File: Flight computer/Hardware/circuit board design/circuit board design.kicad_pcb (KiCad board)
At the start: 4 copper layers, 30.5 x 82.6 mm, 91 parts, among them J1 Conn_01x05, J2 USB_B_Micro, J3 Screw_Terminal_01x04, J4 Conn_01x02, J5 Screw_Terminal_01x04, J6 Conn_Coaxial, J7 Conn_Coaxial, SW1 SW_DPST, U1 IIS2MDC, U10 BMI088, U11 ATSAML21J18B-AUT, U14 MAX40200AUK, U15 LD3985G33R_TSOT23, U2 0433BM41A0019E, U3 Si4463, U4 MAX-M8C, U5 Si7232DN, U6 Si7232DN, U7 W74M64FV, U8 MS5607-02BA, U9 STF202-22T1G, X1 TM-32.000-AF3-33-S-Oscillator, Y3 16MHz

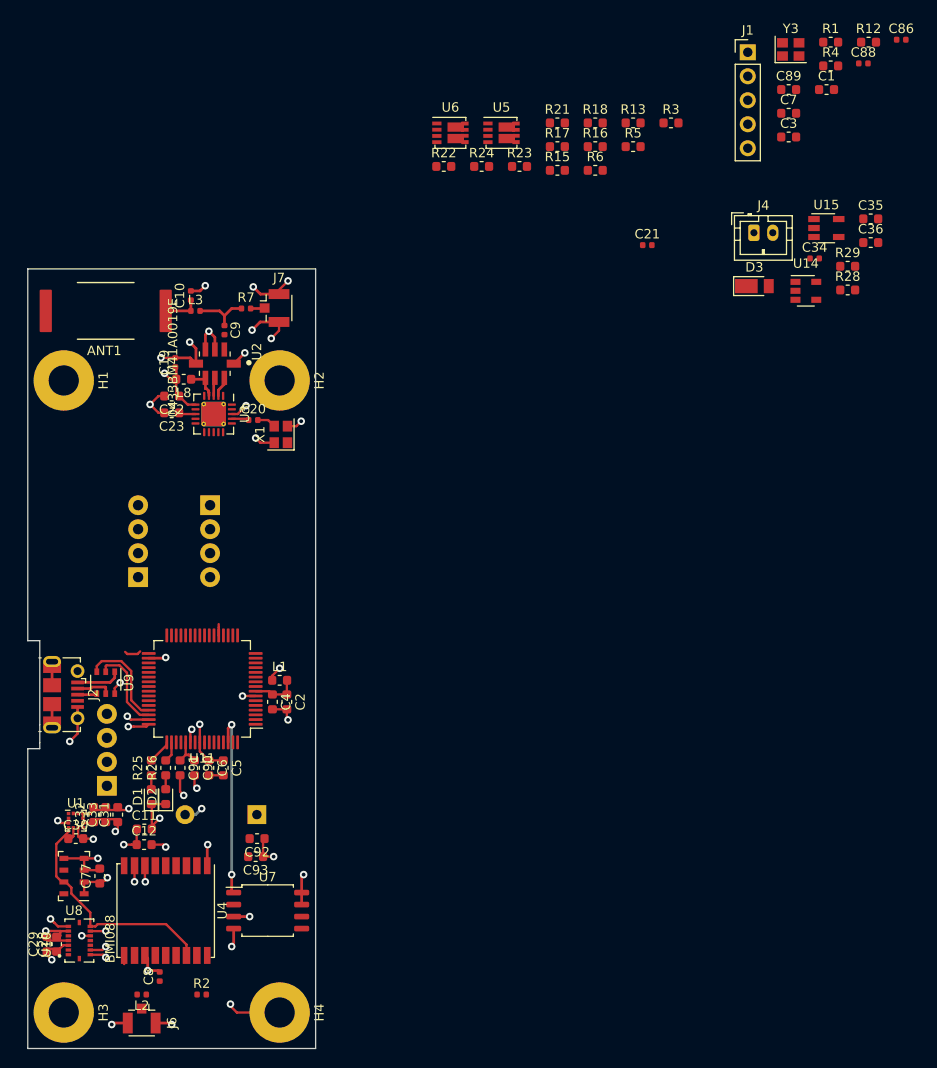
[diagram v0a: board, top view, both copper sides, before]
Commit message: Done extensive routing of the board.
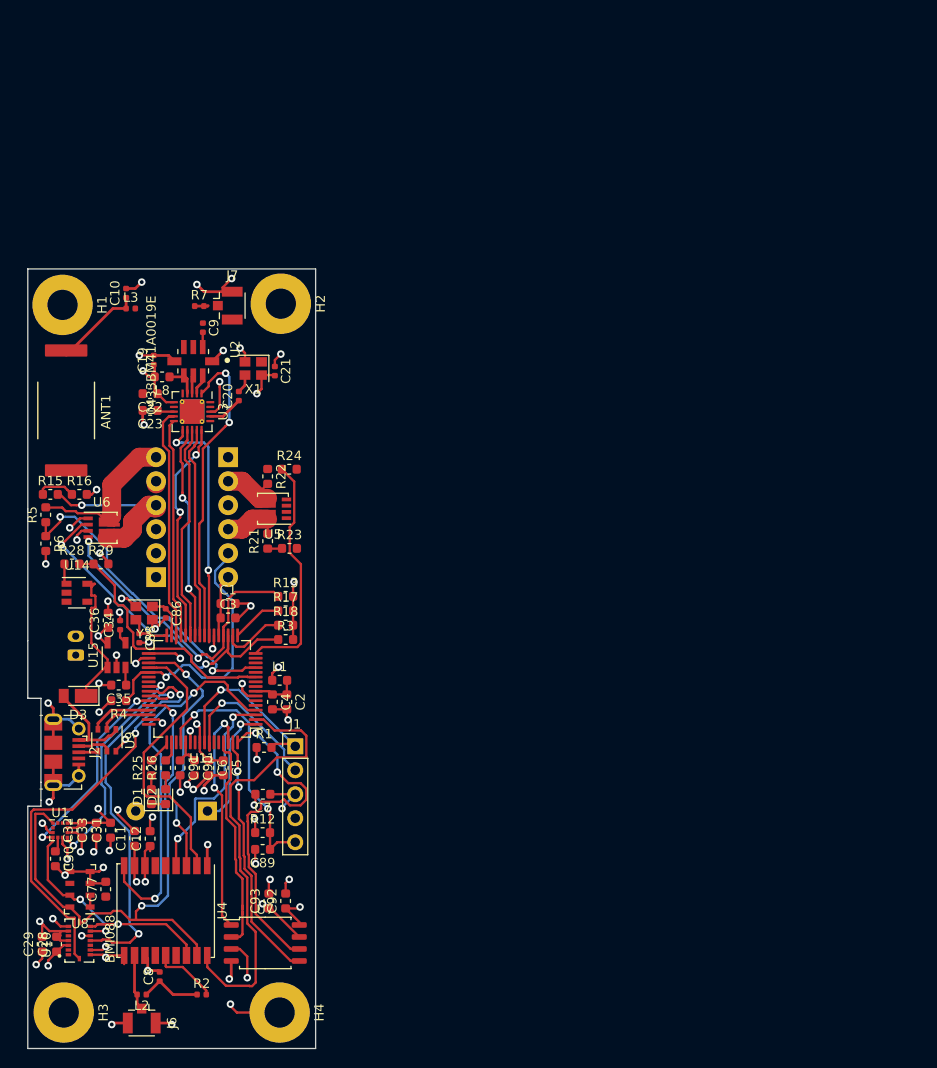
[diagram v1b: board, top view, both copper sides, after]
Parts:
- removed SW1: SW_DPST, flight-computer:TerminalBlock_TE_282834-4_1x04_P2.54mm_Horizontal
- J3, J5: value Screw_Terminal_01x04 -> Screw_Terminal_01x06; footprint flight-computer:TerminalBlock_TE_282834-4_1x04_P2.54mm_Horizontal -> flight-computer:TerminalBlock_TE_282834-6_1x06_P2.54mm_Horizontal
- J4: moved to B.Cu
- moved R12 105.5 mm to (276.3, 306.1)
- moved R4 101.0 mm to (261.1, 292.1), turned to 180 degrees
- moved C86 98.8 mm to (266.1, 282.9), turned to 270 degrees
- moved C88 97.9 mm to (263.3, 285.5), turned to 270 degrees
- moved C89 97.9 mm to (276.3, 307.8), turned to 180 degrees
- moved R1 95.8 mm to (276.5, 297.1)
- moved C35 93.7 mm to (261.1, 290.4), turned to 180 degrees
- moved C7 91.1 mm to (276.4, 302.0), turned to 180 degrees
- moved Y3 90.8 mm to (263.8, 282.8), turned to 180 degrees
- moved C36 90.1 mm to (260.0, 283.6), turned to 90 degrees
- moved J1 87.7 mm to (279.8, 296.9)
- moved U15 87.7 mm to (260.9, 287.3), turned to 90 degrees
- moved R28 87.1 mm to (256.1, 277.6)
- moved R29 85.1 mm to (259.2, 277.6)
- moved J4 84.6 mm to (256.5, 287.3), turned to 90 degrees
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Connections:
- ANT1 pad 2: Net-(ANT1-Pad2) -> (no net)
- J2 pad 4: Net-(J2-Pad4) -> (no net)
- J3 pad 2: /pyro_driver/FET_B -> Vdrive
- J3 pad 4: /pyro_driver/FET_A -> /pyro_driver/FET_B
- U1 pad 11: Net-(U1-Pad11) -> (no net)
- U1 pad 12: Net-(U1-Pad12) -> (no net)
- U1 pad 2: Net-(U1-Pad2) -> (no net)
- U10 pad 1: Net-(U10-Pad1) -> (no net)
- U10 pad 13: Net-(U10-Pad13) -> (no net)
- U10 pad 5: Net-(U10-Pad5) -> (no net)
- U11 pad 10: Net-(U11-Pad10) -> (no net)
- U11 pad 12: Net-(U11-Pad12) -> (no net)
- U11 pad 17: /pyro_driver/FIRE_A -> /pyro_driver/FIRE_C
- U11 pad 18: /pyro_driver/FIRE_B -> /pyro_driver/FIRE_D
- U11 pad 19: /pyro_driver/FIRE_C -> /pyro_driver/FIRE_A
- U11 pad 20: /pyro_driver/FIRE_D -> /pyro_driver/FIRE_B
- U11 pad 38: Net-(U11-Pad38) -> (no net)
- U11 pad 39: Net-(U11-Pad39) -> (no net)
- U11 pad 5: Net-(U11-Pad5) -> (no net)
- U11 pad 51: Net-(U11-Pad51) -> (no net)
- U11 pad 55: Net-(U11-Pad55) -> (no net)
- U11 pad 59: Net-(U11-Pad59) -> (no net)
- U11 pad 6: Net-(U11-Pad6) -> (no net)
- U11 pad 60: Net-(U11-Pad60) -> (no net)
- U11 pad 9: Net-(U11-Pad9) -> (no net)
- U14 pad 4: Net-(U14-Pad4) -> (no net)
- U3 pad 10: /MCU/MCU_PA13 -> /MCU/MCU_PA12
- U3 pad 16: Net-(U3-Pad16) -> (no net)
- U3 pad 19: Net-(U3-Pad19) -> (no net)
- U3 pad 20: Net-(U3-Pad20) -> (no net)
- U3 pad 5: Net-(U3-Pad5) -> (no net)
- U3 pad 7: Net-(U3-Pad7) -> (no net)
- U3 pad 9: /MCU/MCU_PA12 -> /MCU/MCU_PA13
- U4 pad 13: Net-(U4-Pad13) -> (no net)
- U4 pad 15: Net-(U4-Pad15) -> (no net)
- U4 pad 5: Net-(U4-Pad5) -> (no net)
- U4 pad 6: Net-(U4-Pad6) -> (no net)
- U8 pad 6: Net-(U8-Pad6) -> (no net)
- X1 pad 1: Net-(X1-Pad1) -> (no net)
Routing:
- net Net-(J3-Pad1): track 0.00 -> 162.0 mm
- net /gps/GPS_SCL: track 0.20 -> 59.6 mm, vias 0 -> 2
- net /gps/GPS_NSAFEBOOT: track 0.00 -> 46.9 mm
- net /sensors/ACCL_RDY: track 0.00 -> 44.5 mm, vias 0 -> 2
- net GND: track 106.6 -> 150.8 mm, vias 35 -> 58
- net /gps/GPS_NRES: track 0.00 -> 39.6 mm, vias 0 -> 2
- net /sensors/GYRO_RDY: track 0.00 -> 38.6 mm, vias 0 -> 2
- net /pyro_driver/FIRE_A: track 0.00 -> 38.2 mm, vias 0 -> 2
- net /MCU/MCU_SCLK4: track 0.00 -> 37.1 mm, vias 0 -> 2
- net /MCU/MCU_PA04: track 0.00 -> 34.3 mm, vias 0 -> 2
- net /MCU/MCU_PB11: track 0.00 -> 33.1 mm, vias 0 -> 2
- net /pyro_driver/FIRE_B: track 0.00 -> 32.9 mm, vias 0 -> 2
- net /MCU/GPS_RXD0: track 0.00 -> 29.4 mm
- net /MCU/ARMED: track 0.00 -> 28.8 mm, vias 0 -> 1
- net Net-(C89-Pad1): track 0.00 -> 27.6 mm, vias 0 -> 2
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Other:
- outline, holes or cut-outs redrawn
